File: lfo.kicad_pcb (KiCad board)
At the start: 2 copper layers, 103.7 x 33.7 mm, 34 parts, among them J1 PJ398SM-12 (Tri), J2 PJ398SM-12 (square), J3 PJ398SM-12 (weird), J4 Conn_02x05_Odd_Even, Q1 BC547, SW1 SW_SPDT, U1 TL084

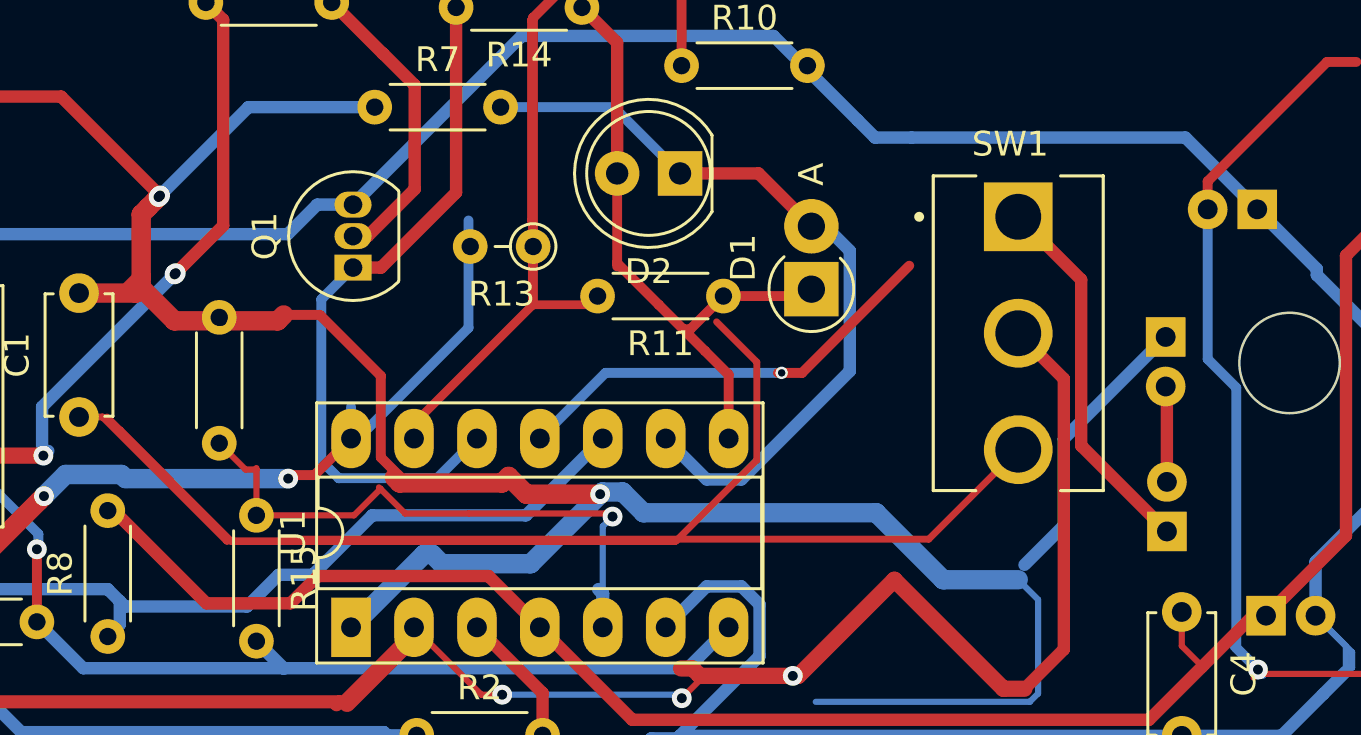
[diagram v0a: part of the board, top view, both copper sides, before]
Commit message: finalize
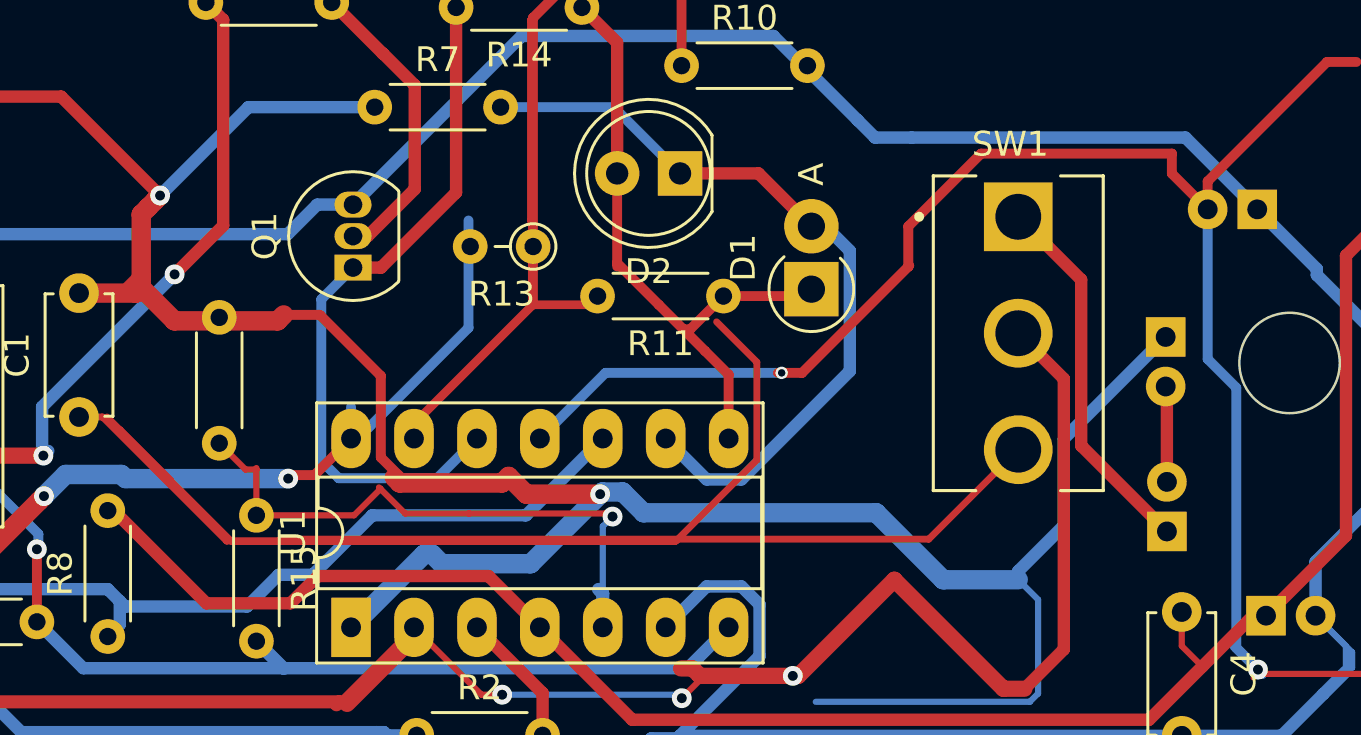
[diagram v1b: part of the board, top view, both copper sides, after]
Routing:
- net Vee: track 55.1 -> 71.4 mm
- net Net-(C1-Pad2): track 121.2 -> 121.9 mm, vias 4 -> 2
- net Net-(R15-Pad2): track 109.5 -> 109.4 mm, vias 4 -> 3
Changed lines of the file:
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@@
+	)
+	(segment
+		(start 132.111883 22.538117)
+		(end 135.05 19.6)
+		(width 0.4)
+		(layer "F.Cu")
+		(net 2)
+	)
+	(segment
+		(start 142.75 19.6)
+		(end 142.75 20.405112)
+		(width 0.4)
+		(layer "F.Cu")
+		(net 2)
 	)
 	(segment
@@
 	)
 	(segment
+		(start 132.111883 24.161883)
+		(end 127.823766 28.45)
+		(width 0.4)
+		(layer "F.Cu")
+		(net 2)
+	)
+	(segment
 		(start 150.195 15.9)
 		(end 149.013518 15.9)
@@
 	)
 	(segment
+		(start 142.75 20.405112)
+		(end 144.194888 21.85)
+		(width 0.4)
+		(layer "F.Cu")
+		(net 2)
+	)
+	(segment
 		(start 132.15 24.123766)
-		(end 127.823766 28.45)
+		(end 132.111883 24.161883)
 		(width 0.4)
 		(layer "F.Cu")
@@
 	)
 	(segment
+		(start 132.111883 24.161883)
+		(end 132.111883 22.538117)
+		(width 0.4)
+		(layer "F.Cu")
+		(net 2)
+	)
+	(segment
 		(start 127.823766 28.45)
 		(end 127 28.45)
+		(width 0.4)
+		(layer "F.Cu")
+		(net 2)
+	)
+	(segment
+		(start 135.05 19.6)
+		(end 142.75 19.6)
 		(width 0.4)
 		(layer "F.Cu")
@@
 	)
 	(via
-		(at 104.4 26.35)
-		(size 0.8)
-		(drill 0.4)
-		(layers "F.Cu" "B.Cu")
-		(net 5)
-	)
-	(via
 		(at 101.91198 21.29198)
 		(size 0.8)
@@
 		(net 5)
 	)
-	(via
-		(at 101.850964 21.352995)
-		(size 0.8)
-		(drill 0.4)
-		(layers "F.Cu" "B.Cu")
-		(net 5)
-	)
 	(segment
 		(start 105.478959 17.725)
@@
 	)
 	(segment
+		(start 136.55 36.45)
+		(end 136.55 36.8)
+		(width 0.5)
+		(layer "B.Cu")
+		(net 5)
+	)
+	(segment
 		(start 130.81611 34.09611)
 		(end 133.52 36.8)
@@
 		(end 112.9 35.775)
 		(width 0.7834)
+		(layer "B.Cu")
+		(net 5)
+	)
+	(segment
+		(start 138.3885 34.6115)
+		(end 136.55 36.45)
+		(width 0.5)
 		(layer "B.Cu")
 		(net 5)
@@
 	)
 	(segment
-		(start 138.3885 34.6115)
-		(end 136.8 36.2)
-		(width 0.5)
-		(layer "B.Cu")
-		(net 5)
-	)
-	(segment
 		(start 109.62 38.72)
 		(end 109.790425 38.72)
@@
 		(start 102.4975 24.4725)
 		(end 102.47 24.5)
-		(width 0.5)
-		(layer "F.Cu")
-		(net 9)
-	)
-	(segment
-		(start 102.545 24.425)
-		(end 102.4975 24.4725)
 		(width 0.5)
 		(layer "F.Cu")
@@
 		(size 0.8)
 		(drill 0.4)
-		(layers "F.Cu" "B.Cu")
-		(net 9)
-	)
-	(via
-		(at 102.545 24.425)
-		(size 0.8)
-		(drill 0.4)
